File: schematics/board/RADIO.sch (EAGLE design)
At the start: 2 parts

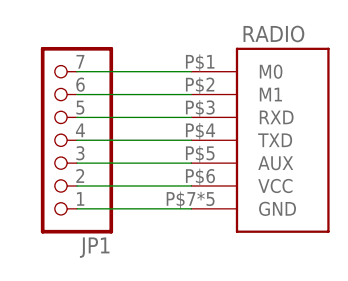
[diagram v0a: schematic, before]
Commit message: Платы подготовлены для Резонита
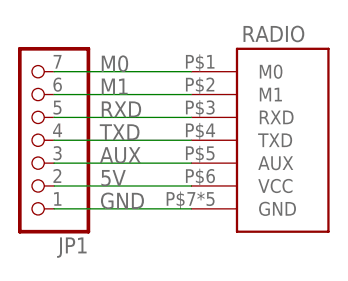
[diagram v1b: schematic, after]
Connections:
- net N$1 renamed GND
- net N$2 renamed 5V
- net N$3 renamed AUX
- net N$4 renamed TXD
- net N$5 renamed RXD
- net N$6 renamed M1
- net N$7 renamed M0
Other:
- moved on the sheet: JP1
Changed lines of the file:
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@@
 <?xml version="1.0" encoding="utf-8"?>
 <!DOCTYPE eagle SYSTEM "eagle.dtd">
-<eagle version="9.6.0">
+<eagle version="9.4.2">
 <drawing>
 <settings>
@@
 <attribute name="NAME" x="5.588" y="31.242" size="1.778" layer="95"/>
 </instance>
-<instance part="JP1" gate="A" x="-15.24" y="20.32" smashed="yes" rot="R180">
-<attribute name="NAME" x="-8.89" y="9.525" size="1.778" layer="95" rot="R180"/>
-<attribute name="VALUE" x="-8.89" y="33.02" size="1.778" layer="96" rot="R180"/>
+<instance part="JP1" gate="A" x="-17.78" y="20.32" smashed="yes" rot="R180">
+<attribute name="NAME" x="-11.43" y="9.525" size="1.778" layer="95" rot="R180"/>
+<attribute name="VALUE" x="-11.43" y="33.02" size="1.778" layer="96" rot="R180"/>
 </instance>
 </instances>
@@
 </busses>
 <nets>
-<net name="N$1" class="0">
+<net name="GND" class="0">
 <segment>
 <pinref part="RADIO" gate="G$1" pin="GND"/>
 <pinref part="JP1" gate="A" pin="1"/>
-<wire x1="-12.7" y1="12.7" x2="0" y2="12.7" width="0.1524" layer="91"/>
+<wire x1="-15.24" y1="12.7" x2="0" y2="12.7" width="0.1524" layer="91"/>
+<label x="-10.16" y="12.7" size="1.778" layer="95"/>
 </segment>
 </net>
-<net name="N$2" class="0">
+<net name="5V" class="0">
 <segment>
 <pinref part="RADIO" gate="G$1" pin="VCC"/>
 <pinref part="JP1" gate="A" pin="2"/>
-<wire x1="-12.7" y1="15.24" x2="0" y2="15.24" width="0.1524" layer="91"/>
+<wire x1="-15.24" y1="15.24" x2="0" y2="15.24" width="0.1524" layer="91"/>
+<label x="-10.16" y="15.24" size="1.778" layer="95"/>
 </segment>
 </net>
-<net name="N$3" class="0">
+<net name="AUX" class="0">
 <segment>
 <pinref part="RADIO" gate="G$1" pin="AUX"/>
 <pinref part="JP1" gate="A" pin="3"/>
-<wire x1="-12.7" y1="17.78" x2="0" y2="17.78" width="0.1524" layer="91"/>
+<wire x1="-15.24" y1="17.78" x2="0" y2="17.78" width="0.1524" layer="91"/>
+<label x="-10.16" y="17.78" size="1.778" layer="95"/>
 </segment>
 </net>
-<net name="N$4" class="0">
+<net name="TXD" class="0">
 <segment>
 <pinref part="RADIO" gate="G$1" pin="TXD"/>
 <pinref part="JP1" gate="A" pin="4"/>
-<wire x1="-12.7" y1="20.32" x2="0" y2="20.32" width="0.1524" layer="91"/>
+<wire x1="-15.24" y1="20.32" x2="0" y2="20.32" width="0.1524" layer="91"/>
+<label x="-10.16" y="20.32" size="1.778" layer="95"/>
 </segment>
 </net>
-<net name="N$5" class="0">
+<net name="RXD" class="0">
 <segment>
 <pinref part="RADIO" gate="G$1" pin="RXD"/>
 <pinref part="JP1" gate="A" pin="5"/>
-<wire x1="-12.7" y1="22.86" x2="0" y2="22.86" width="0.1524" layer="91"/>
+<wire x1="-15.24" y1="22.86" x2="0" y2="22.86" width="0.1524" layer="91"/>
+<label x="-10.16" y="22.86" size="1.778" layer="95"/>
 </segment>
 </net>
-<net name="N$6" class="0">
+<net name="M1" class="0">
 <segment>
 <pinref part="RADIO" gate="G$1" pin="M1"/>
 <pinref part="JP1" gate="A" pin="6"/>
-<wire x1="-12.7" y1="25.4" x2="0" y2="25.4" width="0.1524" layer="91"/>
+<wire x1="-15.24" y1="25.4" x2="0" y2="25.4" width="0.1524" layer="91"/>
+<label x="-10.16" y="25.4" size="1.778" layer="95"/>
 </segment>
 </net>
-<net name="N$7" class="0">
+<net name="M0" class="0">
 <segment>
 <pinref part="RADIO" gate="G$1" pin="M0"/>
 <pinref part="JP1" gate="A" pin="7"/>
-<wire x1="-12.7" y1="27.94" x2="0" y2="27.94" width="0.1524" layer="91"/>
+<wire x1="-15.24" y1="27.94" x2="0" y2="27.94" width="0.1524" layer="91"/>
+<label x="-10.16" y="27.94" size="1.778" layer="95"/>
 </segment>
 </net>
